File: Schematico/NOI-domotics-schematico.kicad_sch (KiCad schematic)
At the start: 4 parts

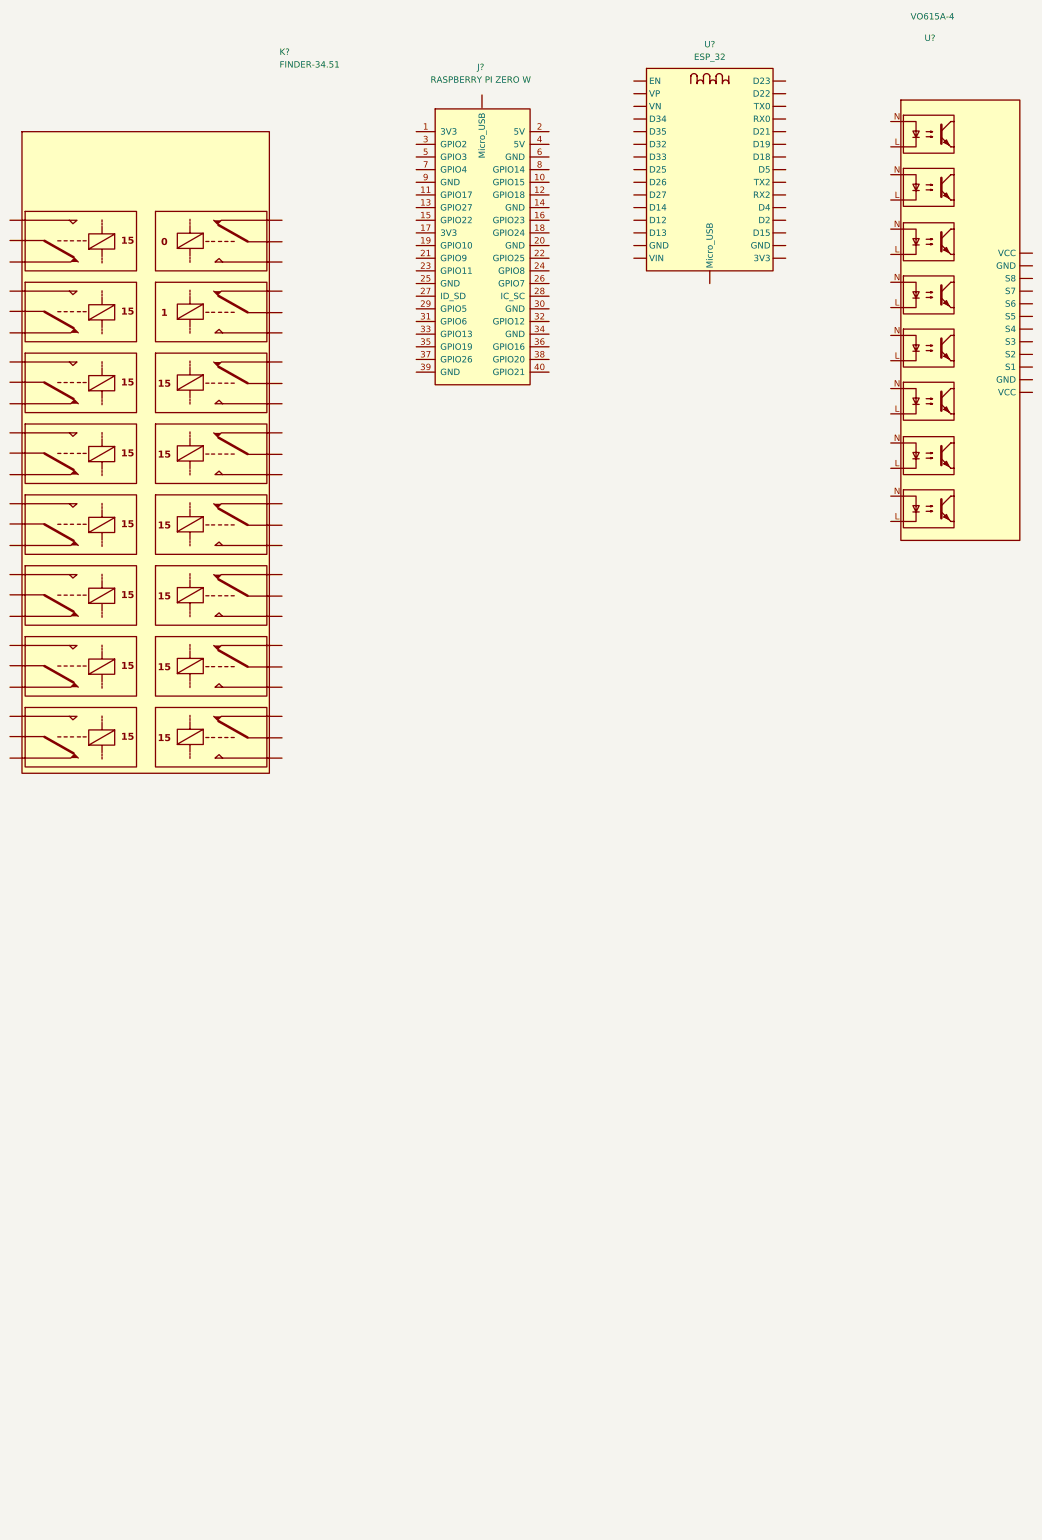
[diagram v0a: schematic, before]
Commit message: avanzo
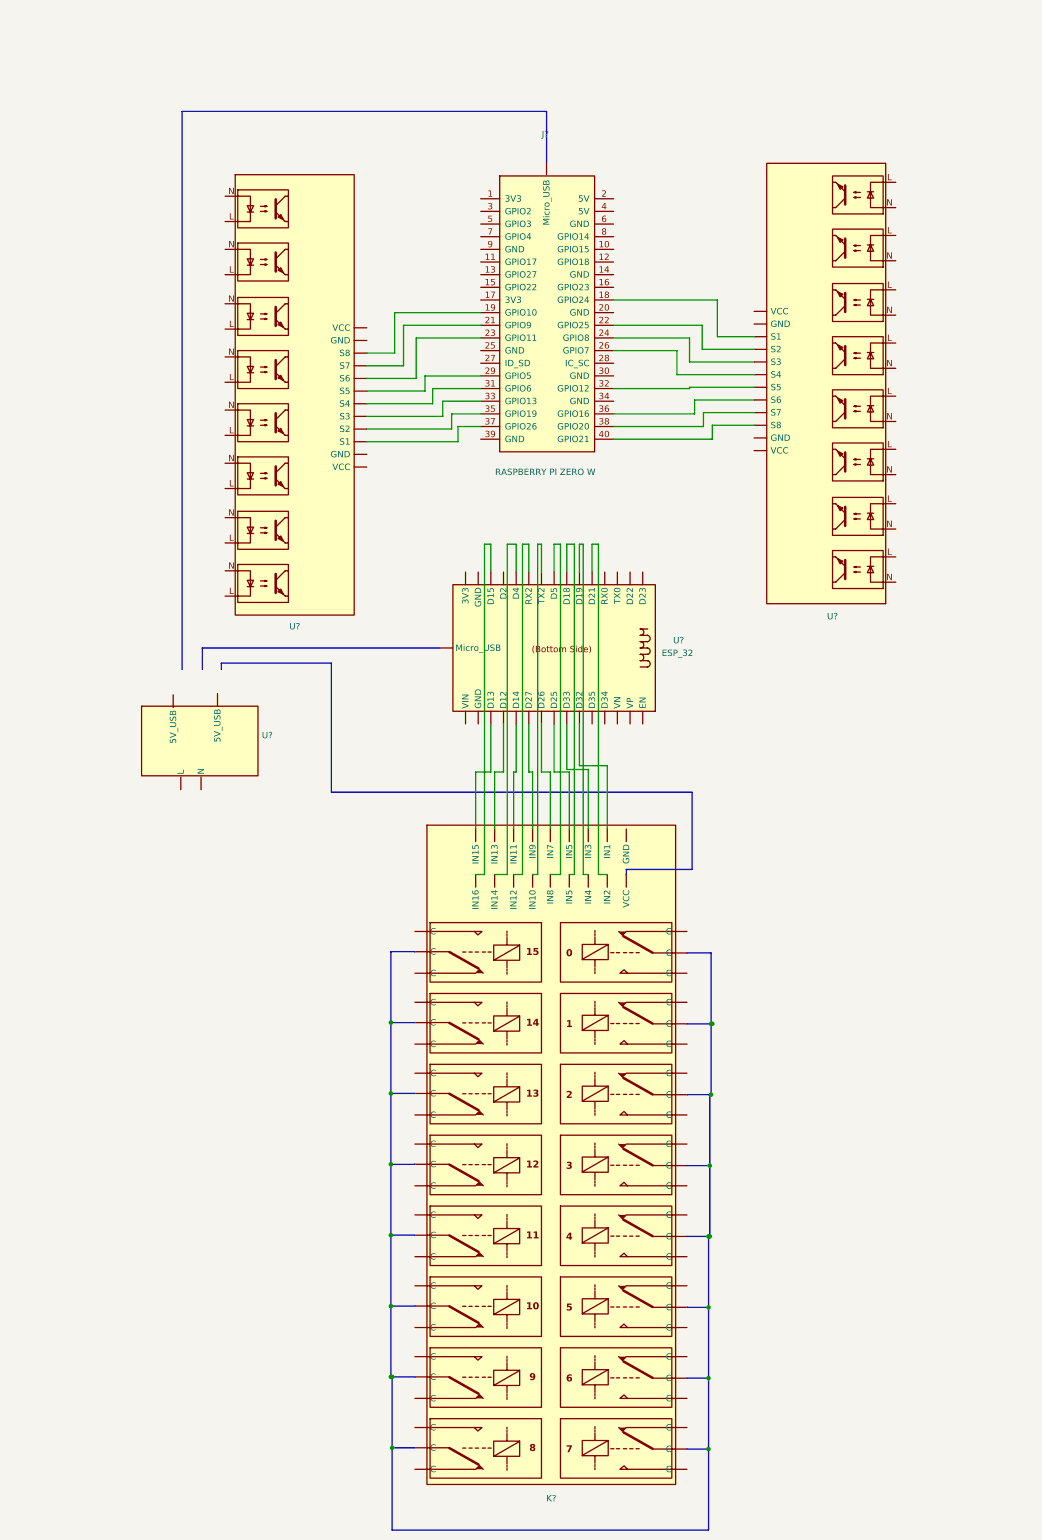
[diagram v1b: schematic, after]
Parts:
- added U?: (no value), symbol USB_5V:USB_DCconverter
- added U?: (no value), symbol Isolator:VO615A-4
- K?: value FINDER-34.51 -> (none)
- U?: value VO615A-4 -> (none)
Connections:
- net at U?. (VCC): now also J?.37 (GPIO26)
- net at J?.18 (GPIO24): now also U?. (VCC)
- net at J?.19 (GPIO10): now also U?. (VCC)
- net at J?.21 (GPIO9): now also U?. (VCC)
- net at J?.22 (GPIO25): now also U?. (VCC)
- net at J?.23 (GPIO11): now also U?. (VCC)
- net at J?.24 (GPIO8): now also U?. (VCC)
- net at J?.26 (GPIO7): now also U?. (VCC)
- net at J?.29 (GPIO5): now also U?. (VCC)
- net at J?.31 (GPIO6): now also U?. (VCC)
- net at J?.32 (GPIO12): now also U?. (VCC)
- net at J?.33 (GPIO13): now also U?. (VCC)
- net at J?.35 (GPIO19): now also U?. (VCC)
- net at J?.36 (GPIO16): now also U?. (VCC)
- net at J?.38 (GPIO20): now also U?. (VCC)
- net at J?.40 (GPIO21): now also U?. (VCC)
- net at K?. (VCC): now also U?.1 (VP)
- new net: K?. (VCC), U?.1 (VP) (x15)
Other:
- moved on the sheet: J?, U?
